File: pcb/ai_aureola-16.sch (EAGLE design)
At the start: 29 parts

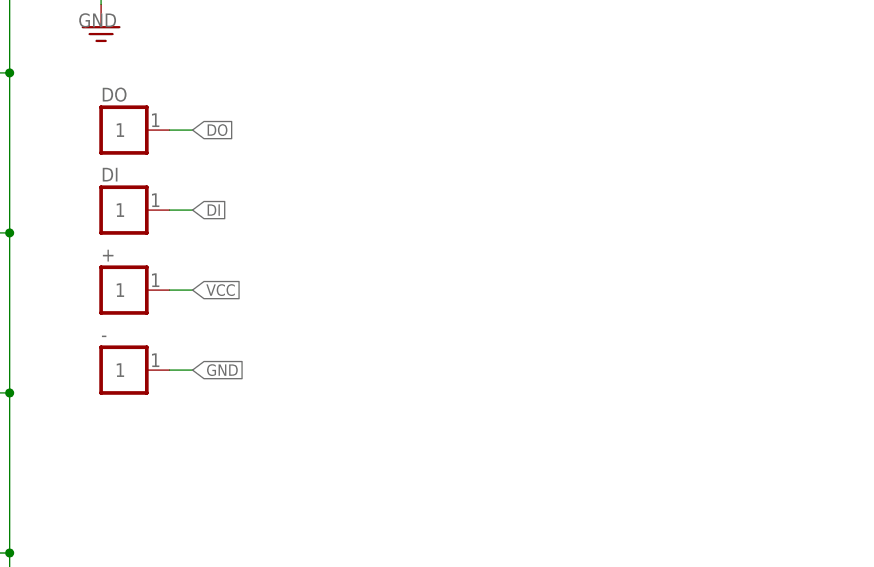
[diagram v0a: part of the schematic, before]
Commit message: ready for manufacturing
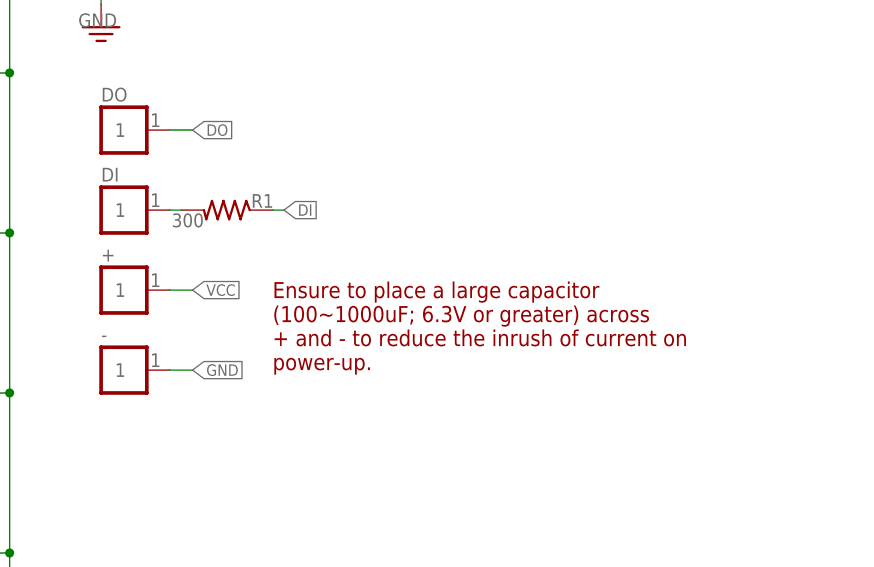
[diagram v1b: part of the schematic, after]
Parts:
- added R1: 300, Ai_Passives:RES0402
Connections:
- new net N$3: DI.1, R1.2
- net DI: now also R1.1; no longer DI.1
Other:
- note added: "Ensure to place a large capacitor (100~1000uF; 6.3V or greater) across + and - to reduce the inrush of current on power-up."
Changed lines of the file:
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@@
 <part name="-" library="Ai_Connectors" deviceset="1X01" device="-SM" value="1X01-SM"/>
 <part name="LOGO" library="Ai_Miscellany" deviceset="AI-LOGO" device="XS"/>
+<part name="R1" library="Ai_Passives" deviceset="RES" device="0402" value="300"/>
 </parts>
 <sheets>
 <sheet>
 <plain>
+<text x="120.65" y="119.38" size="1.778" layer="94">Ensure to place a large capacitor
+(100~1000uF; 6.3V or greater) across
++ and - to reduce the inrush of current on
+power-up.</text>
 </plain>
 <instances>
@@
 <instance part="-" gate="G$1" x="104.14" y="119.38"/>
 <instance part="LOGO" gate="G$1" x="138.43" y="12.7"/>
+<instance part="R1" gate="G$1" x="115.57" y="137.16" rot="MR0"/>
 </instances>
 <busses>
@@
 </segment>
 <segment>
-<pinref part="DI" gate="G$1" pin="1"/>
-<wire x1="109.22" y1="137.16" x2="111.76" y2="137.16" width="0.1524" layer="91"/>
-<label x="111.76" y="137.16" size="1.27" layer="95" font="vector" ratio="15" xref="yes"/>
+<pinref part="R1" gate="G$1" pin="1"/>
+<wire x1="120.65" y1="137.16" x2="121.92" y2="137.16" width="0.1524" layer="91"/>
+<label x="121.92" y="137.16" size="1.27" layer="95" font="vector" ratio="15" xref="yes"/>
 </segment>
 </net>
@@
 </segment>
 </net>
+<net name="N$3" class="0">
+<segment>
+<pinref part="R1" gate="G$1" pin="2"/>
+<pinref part="DI" gate="G$1" pin="1"/>
+<wire x1="110.49" y1="137.16" x2="109.22" y2="137.16" width="0.1524" layer="91"/>
+</segment>
+</net>
 </nets>
 </sheet>
@@
 </schematic>
 </drawing>
+<compatibility>
+<note version="6.3" minversion="6.2.2" severity="warning">
+Since Version 6.2.2 text objects can contain more than one line,
+which will not be processed correctly with this version.
+</note>
+</compatibility>
 </eagle>
